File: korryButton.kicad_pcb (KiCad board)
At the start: 2 copper layers, 30 x 30 mm, 15 parts, among them CN1 B2B-XH-A (LF)(SN), CN2 B2B-XH-A (LF)(SN), SW1 5.8 ZSGT, U1 SN74AHCT125DR, U2 B3B-XH-A(LF)(SN), U3 WS2811C, U4 WS2811C

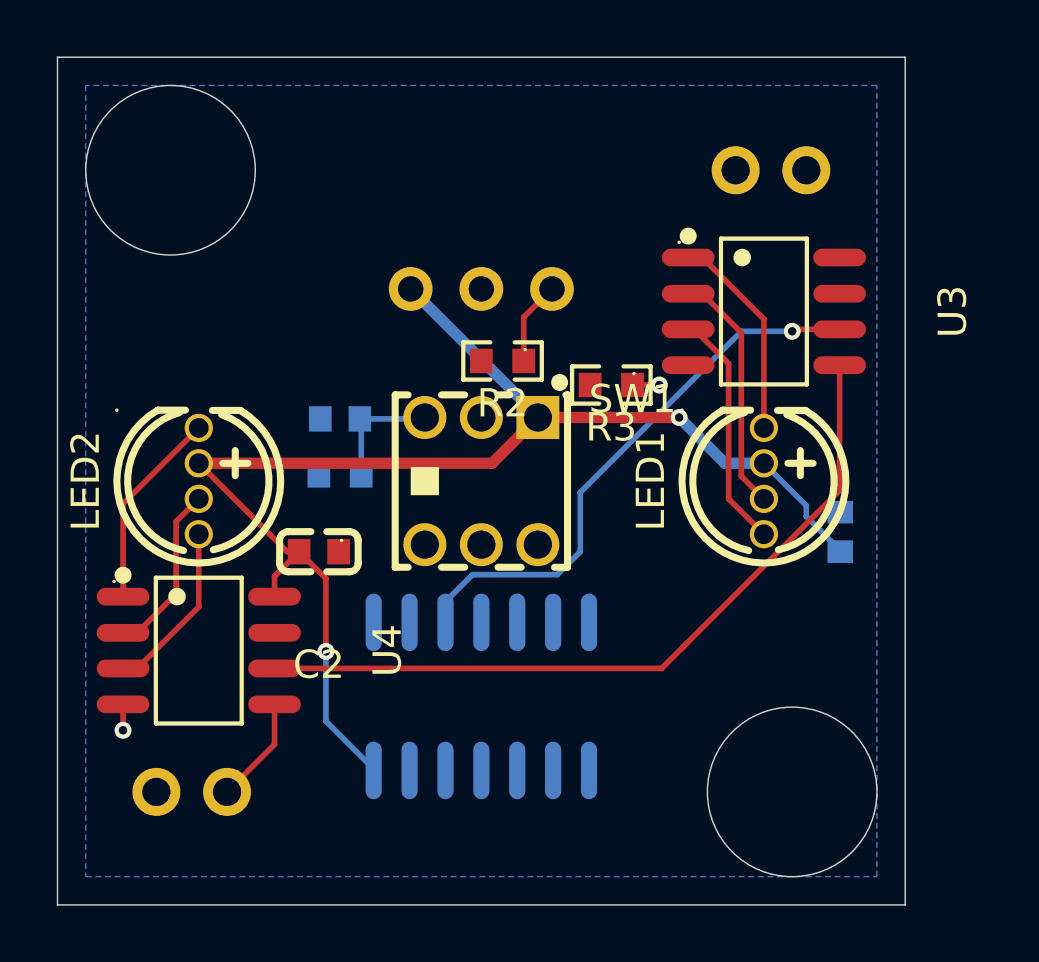
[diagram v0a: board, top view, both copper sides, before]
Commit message: update schematic, pcb
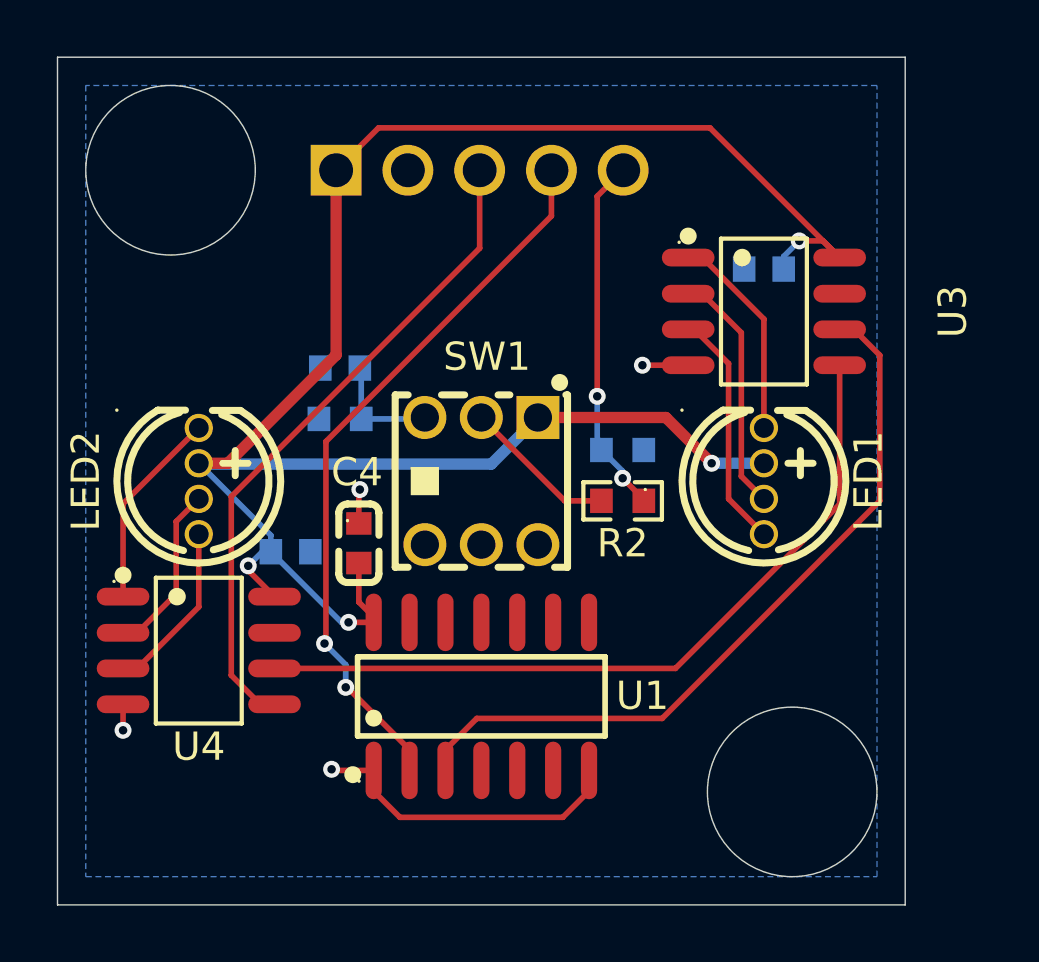
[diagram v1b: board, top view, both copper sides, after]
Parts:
- removed CN2: B2B-XH-A (LF)(SN), lcsc_footprints:C158012_CONN-TH_B2B-XH-A-LF-SN
- removed U2: B3B-XH-A(LF)(SN), lcsc_footprints:C144394_CONN-TH_3P-P2_50_A2501WV2-3P
- added C4: 100nF (104) ±10% 50V, lcsc_footprints:C1591_C0603, F.Cu at (95.7, 127.2)
- C2, R3: moved to B.Cu
- CN1: value B2B-XH-A (LF)(SN) -> B5B-XH-A (LF)(SN); footprint lcsc_footprints:C158012_CONN-TH_B2B-XH-A-LF-SN -> lcsc_footprints:C157991_CONN-TH_B5B-XH-A-LF-SN
- U1: moved to F.Cu
- moved C3 19.5 mm to (93.2, 127.5), turned to 180 degrees
- moved C2 18.7 mm to (110.0, 117.5), turned to 0 degrees
- moved CN1 10.3 mm to (99.9, 114.0)
- moved R2 6.52 mm to (105.0, 125.7)
- moved R3 2.33 mm to (105.0, 123.9)
- moved R1 2.00 mm to (95.0, 122.8)
- moved C1 1.80 mm to (95.0, 121.0)
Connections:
- CN1 pad 1: Net-(U1-1A) -> VCC
- R2 pad 1: Net-(R2-Pad1) -> Net-(CN1-Pad5)
- R3 pad 2: Net-(R2-Pad1) -> Net-(CN1-Pad5)
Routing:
- net Net-(U1-1A): track 0.00 -> 25.8 mm, vias 0 -> 2
- net VCC: track 48.1 -> 72.7 mm, vias 2 -> 4
- net Net-(U4-DO): track 3.80 -> 23.5 mm
- net Net-(CN1-Pad5): track 0.00 -> 13.3 mm, vias 0 -> 2
- net GND: track 1.87 -> 15.1 mm, vias 2 -> 4
- net Net-(U1-1Y): track 19.9 -> 26.7 mm, vias 1 -> 0
- net Net-(R2-Pad2): track 0.00 -> 5.47 mm
- net Net-(R2-Pad1): track 2.96 -> 0.00 mm
